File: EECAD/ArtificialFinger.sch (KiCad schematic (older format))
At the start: 48 parts, among them J1 LI-ION, J2 UART, J3 USB_OTG, Q1 PMOS-GDS, SW1 RESET, U1 LSM6DSM, U2 ESP32-WROVER, U3 LTC3440, U4 SDCARD, U5 MCP73831, U6 FT232R

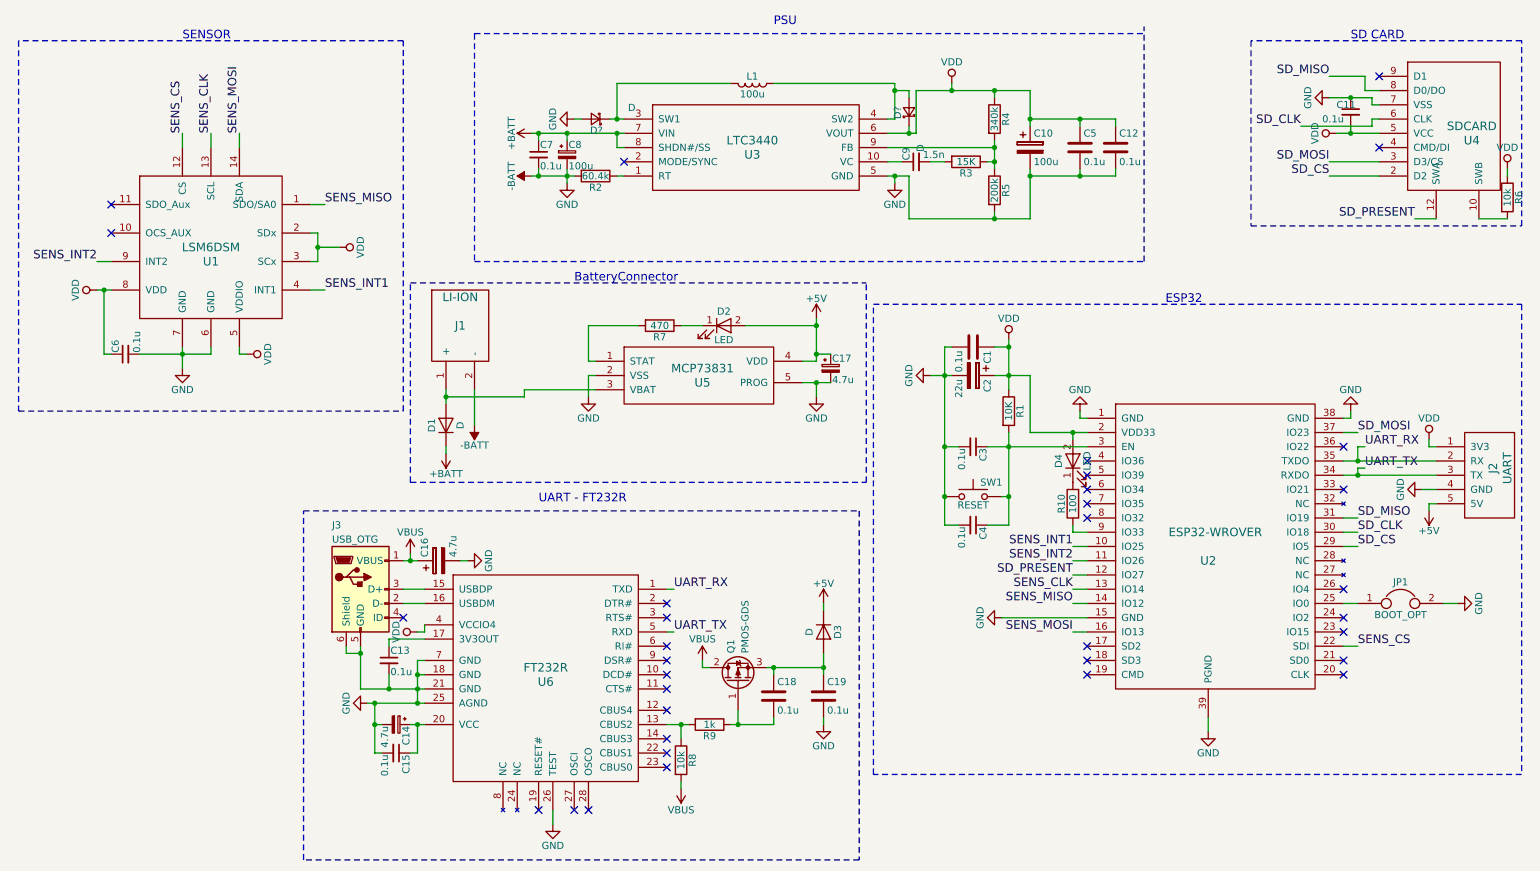
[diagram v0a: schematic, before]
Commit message: Backing up all KiCAD files
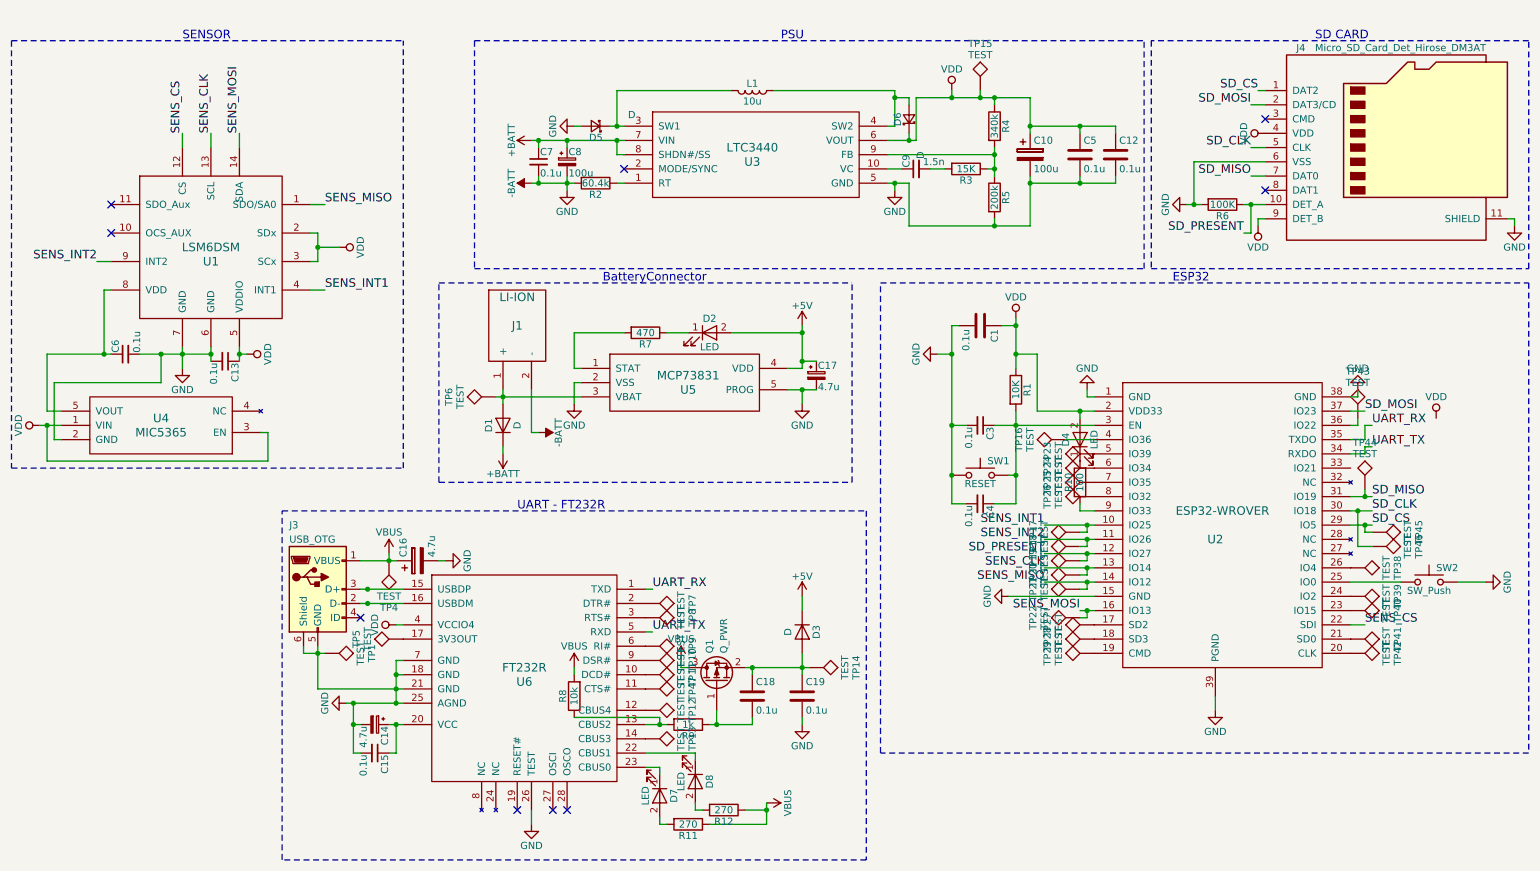
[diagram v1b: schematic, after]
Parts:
- removed C11: 0.1u, Capacitors_SMD:C_0805_HandSoldering, symbol C_Small
- removed C2: 22u, Capacitors_SMD:C_1206_HandSoldering, symbol CP
- removed J2: UART, symbol UART
- removed JP1: BOOT_OPT, symbol Jumper
- removed Q1: PMOS-GDS, symbol Q_PMOS_GDS
- removed U4: SDCARD, symbol SDCARD
- added D7, D8: LED, LEDs:LED_0603_HandSoldering, symbol LED
- added J4: Micro_SD_Card_Det_Hirose_DM3AT, Connectors_Card:Hirose_DM3AT-SF-PEJM5, symbol Micro_SD_Card_Det_Hirose_DM3AT
- added Q1: Q_PWR, TO_SOT_Packages_SMD:SOT-23_Handsoldering, symbol Q_PMOS_GSD
- added R11, R12: 270, Resistors_SMD:R_0805_HandSoldering, symbol R
- added SW2: SW_Push, Buttons_Switches_THT:SW_PUSH_6mm_h4.3mm, symbol SW_Push
- added TP1, TP10, TP11, TP12, TP13, TP14, TP15, TP16, TP17, TP18, TP19, TP20, TP21, TP22, TP23, TP24, TP25, TP26, TP27, TP28, TP29, TP38, TP39, TP4, TP40, TP41, TP42, TP43, TP44, TP45, TP46, TP47, TP5, TP6, TP7, TP8, TP9: TEST, .pretty:TP_SMALL, symbol TEST
- added U4: MIC5365, TO_SOT_Packages_SMD:SOT-23-5_HandSoldering, symbol MIC5365
- C1, C13, C15, C18, C19, C3, C4, C6, C7: footprint Capacitors_SMD:C_0805_HandSoldering -> Capacitors_SMD:C_1206_HandSoldering
- C10, C8: footprint Capacitors_THT:CP_Radial_D6.3mm_P2.50mm -> Capacitors_SMD:CP_Elec_6.3x7.7
- C12, C5: footprint (none) -> Capacitors_SMD:C_1206_HandSoldering
- C9: footprint Capacitors_SMD:C_0805_HandSoldering -> Capacitors_SMD:C_0603_HandSoldering
- D1, D3: footprint (none) -> .pretty:RECTRON_2SS100L
- D2, D4: footprint (none) -> LEDs:LED_0603_HandSoldering
- D5, D6: renamed from D?; footprint (none) -> .pretty:RECTRON_2SS100L
- J1: footprint (none) -> Connectors_JST:JST_PH_S2B-PH-K_02x2.00mm_Angled
- J3: footprint (none) -> .pretty:WurthE_614105150721
- L1: value 100u -> 10u; footprint (none) -> Inductors_THT:L_Axial_L5.3mm_D2.2mm_P10.16mm_Horizontal_Vishay_IM-1
- R1, R2, R3, R4, R5, R7, R8, R9: footprint Capacitors_SMD:C_0805_HandSoldering -> Resistors_SMD:R_0805_HandSoldering
- R10: footprint (none) -> Resistors_SMD:R_0805_HandSoldering
- R6: value 10k -> 100K; footprint Capacitors_SMD:C_0805_HandSoldering -> Resistors_SMD:R_0805_HandSoldering
- SW1: footprint (none) -> Buttons_Switches_THT:SW_PUSH_6mm_h4.3mm
- U1: footprint (none) -> .pretty:LSM6DSM
- U2: footprint (none) -> .pretty:esp32-wrover
- U3: footprint (none) -> Housings_SSOP:MSOP-10_3x3mm_Pitch0.5mm
- U5: footprint (none) -> TO_SOT_Packages_SMD:SOT-23-5
- U6: footprint (none) -> Housings_SSOP:SSOP-28_5.3x10.2mm_Pitch0.65mm
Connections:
- net -BATT: now also R6.2, J4.11 (SHIELD), J4.6 (VSS), SW2.2, TP1.1, U4.2 (GND)
- net SD_CLK: now also J4.5 (CLK), TP46.1
- net SD_CS: now also J4.1 (DAT2), TP45.1
- net SD_MISO: now also J4.7 (DAT0), TP44.1
- net SD_MOSI: now also J4.2 (DAT3/CD)
- net SD_PRESENT: now also R6.1, J4.10 (DET_A), TP19.1
- net SENS_CLK: now also TP20.1
- net SENS_INT1: now also TP17.1
- net SENS_INT2: now also TP18.1
- net SENS_MISO: now also TP21.1
- net SENS_MOSI: now also TP22.1
- net VBUS: now also Q1.3 (D), R11.1, R12.1, TP4.1
- net VDD: now also C13.1, J4.4 (VDD), J4.9 (DET_B), TP15.1, U4.1 (VIN), U4.3 (EN); no longer C6.1, R6.1, U1.8 (VDD)
- net at U2.17 (SD2): now also TP27.1
- net at U2.18 (SD3): now also TP28.1
- net at U2.19 (CMD): now also TP29.1
- net at U2.20 (CLK): now also TP42.1
- net at U2.21 (SD0): now also TP41.1
- net at U2.23 (IO15): now also TP40.1
- net at U2.24 (IO2): now also TP39.1
- net at U2.25 (IO0): now also SW2.1
- net at U2.26 (IO4): now also TP38.1
- net at U2.36 (IO22): now also TP43.1
- net at U2.4 (IO36): now also TP16.1
- net at U2.5 (IO39): now also TP23.1
- net at U2.6 (IO34): now also TP24.1
- net at U2.7 (IO35): now also TP25.1
- net at U2.8 (IO32): now also TP26.1
- net at D1.2 (A), J1.1 (+), U5.3 (VBAT): now also TP6.1
- net at U6.10 (DCD#): now also TP11.1
- net at U6.11 (CTS#): now also TP47.1
- net at U6.12 (CBUS4): now also TP12.1
- net at U6.14 (CBUS3): now also TP13.1
- net at U6.17 (3V3OUT): now also TP5.1; no longer C13.1
- net at U6.2 (DTR#): now also TP7.1
- net at U6.22 (CBUS1): now also D8.1 (K)
- net at U6.23 (CBUS0): now also D7.1 (K)
- net at U6.3 (RTS#): now also TP8.1
- net at U6.6 (RI#): now also TP9.1
- net at U6.9 (DSR#): now also TP10.1
- net at C18.2, R9.1: now also Q1.1 (G)
- net at C18.1, C19.1, D3.2 (A): now also Q1.2 (S), TP14.1
- new net: C6.1, U1.8 (VDD), U4.5 (VOUT)
- new net: D8.2 (A), R12.2
- new net: D7.2 (A), R11.2
- no-connect marks 34 -> 9
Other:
- moved on the sheet: C1, C10, C12, C14, C15, C16, C17, C18, C19, C3, C4, C5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
